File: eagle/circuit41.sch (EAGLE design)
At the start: 18 parts

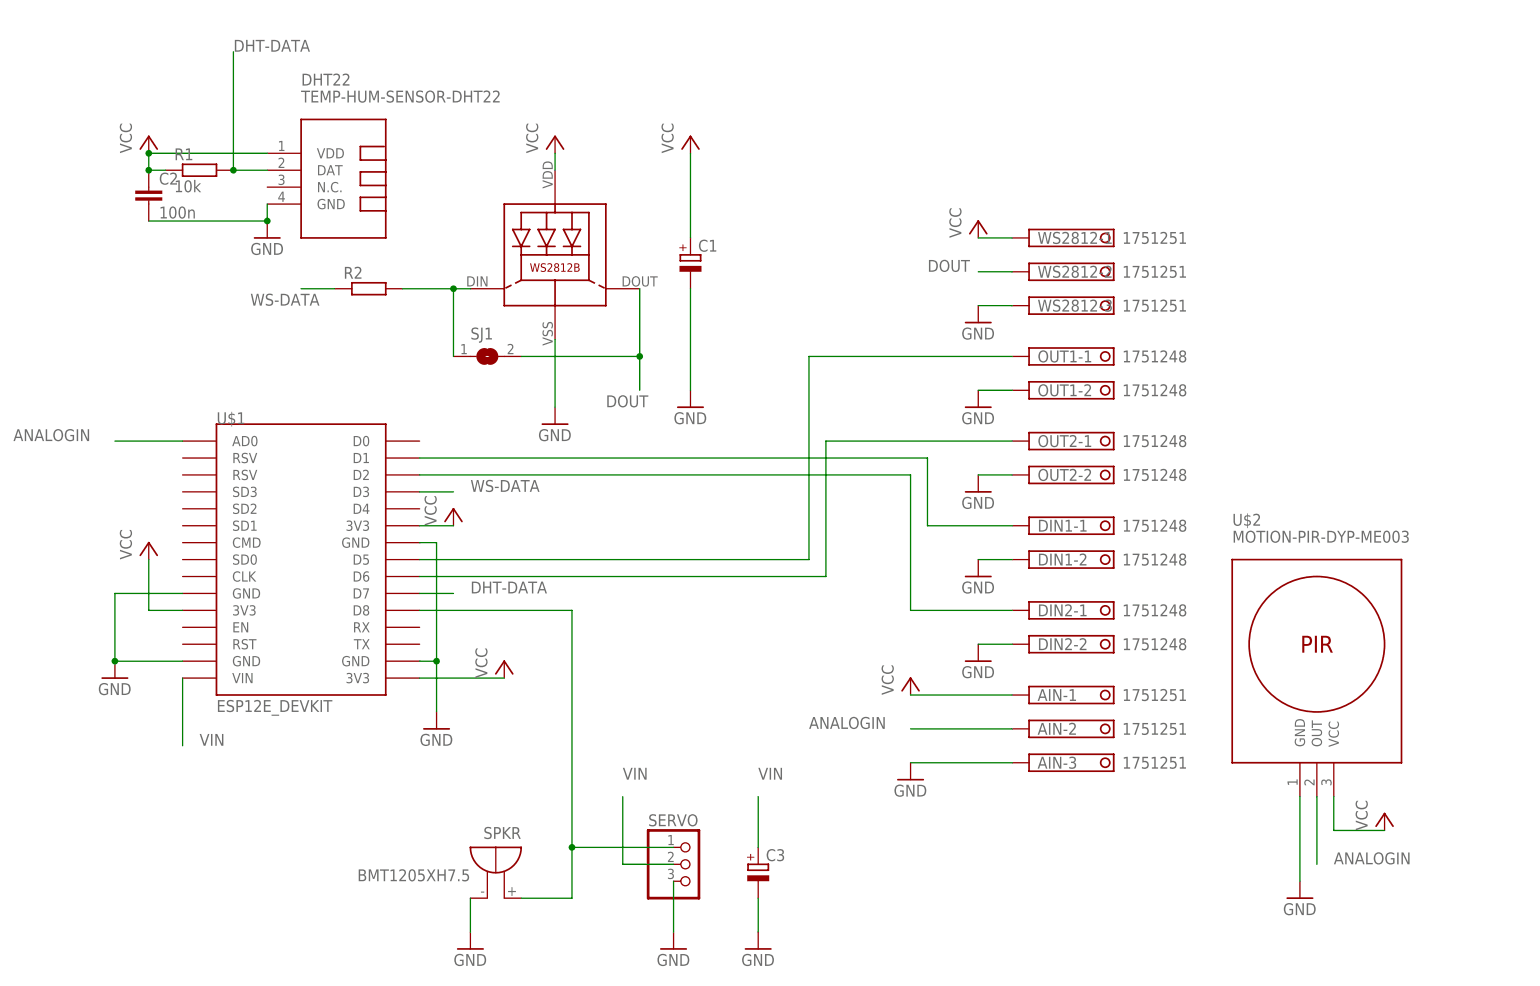
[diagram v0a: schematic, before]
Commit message: main update to version 0.41
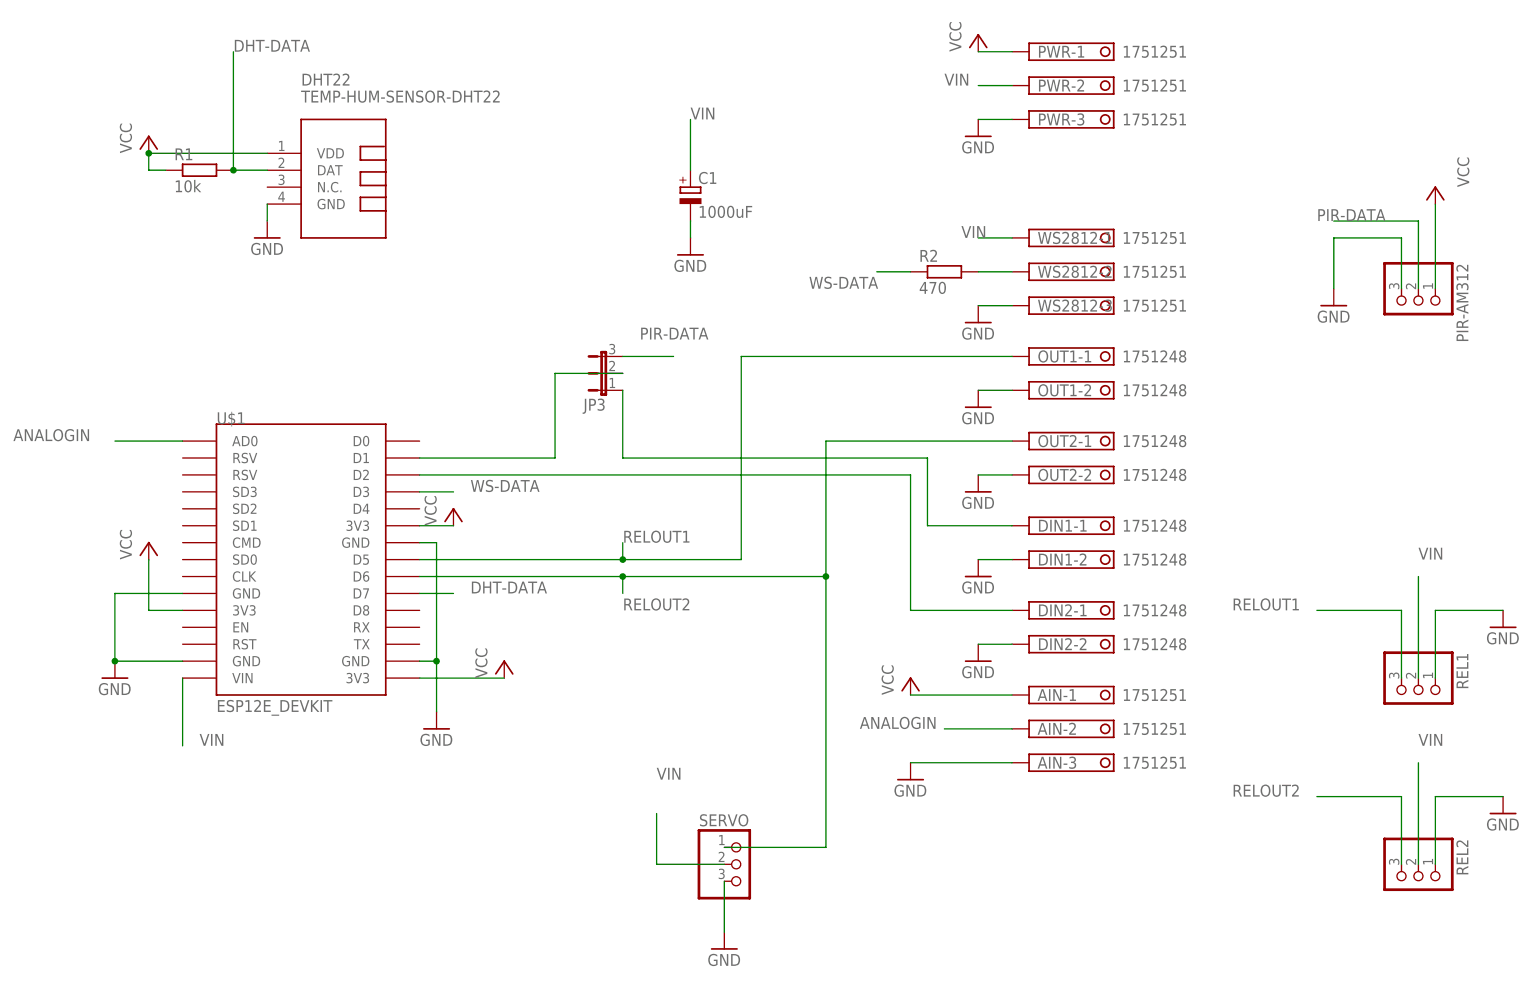
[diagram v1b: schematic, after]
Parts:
- removed C2: 100n, rcl:C-EUC0805
- removed C3: (no value), rcl:CPOL-EUE2.5-7
- removed LED1: WS2812B, WS2812B:WS2812B
- removed SJ1: (no value), jumper:SJ
- removed SPKR: BMT1205XH7.5, buzzer:BMT1205XH7.5
- removed U$2: MOTION-PIR-DYP-ME003, diy-modules:MOTION-PIR-DYP-ME003
- added JP3: (no value), jumper:JP2E
- added PIR-AM312, REL1, REL2: (no value), pinhead:PINHD-1X3
- added PWR: 1751251, con-phoenix-350:1751251
- C1: value (none) -> 1000uF; device rcl:CPOL-EUE2.5-7 -> rcl:CPOL-EUE3.5-8
- R2: value (none) -> 470
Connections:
- removed net N$5: OUT1-1.K, U$1.D5
- removed net N$7: OUT2-1.K, U$1.D6
- removed net N$9: DIN1-1.K, U$1.D1
- removed net WS: LED1.DI, R2.2, SJ1.1
- new net N$2: DIN1-1.K, JP3.1
- new net PIR-DATA: JP3.3, PIR-AM312.2
- new net RELOUT1: OUT1-1.K, REL1.3, U$1.D5
- new net RELOUT2: OUT2-1.K, REL2.3, SERVO.1, U$1.D6
- net ANALOGIN: no longer U$2.OUT
- net DOUT: now also R2.2; no longer LED1.DO, SJ1.2
- net GND: now also PIR-AM312.3, PWR-3.K, REL1.1, REL2.1; no longer C2.2, C3.-, LED1.GND, SPKR.-, U$2.GND
- net N$1: now also JP3.2, U$1.D1; no longer SERVO.1, SPKR.+, U$1.D8
- net VCC: now also PIR-AM312.1, PWR-1.K; no longer C1.+, C2.1, LED1.VDD, U$2.VCC, WS2812-1.K
- net VIN: now also C1.+, PWR-2.K, REL1.2, REL2.2, WS2812-1.K; no longer C3.+
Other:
- moved on the sheet: C1, R2, SERVO
